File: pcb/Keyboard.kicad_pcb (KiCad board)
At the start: 2 copper layers, 158.5 x 92.5 mm, 63 parts

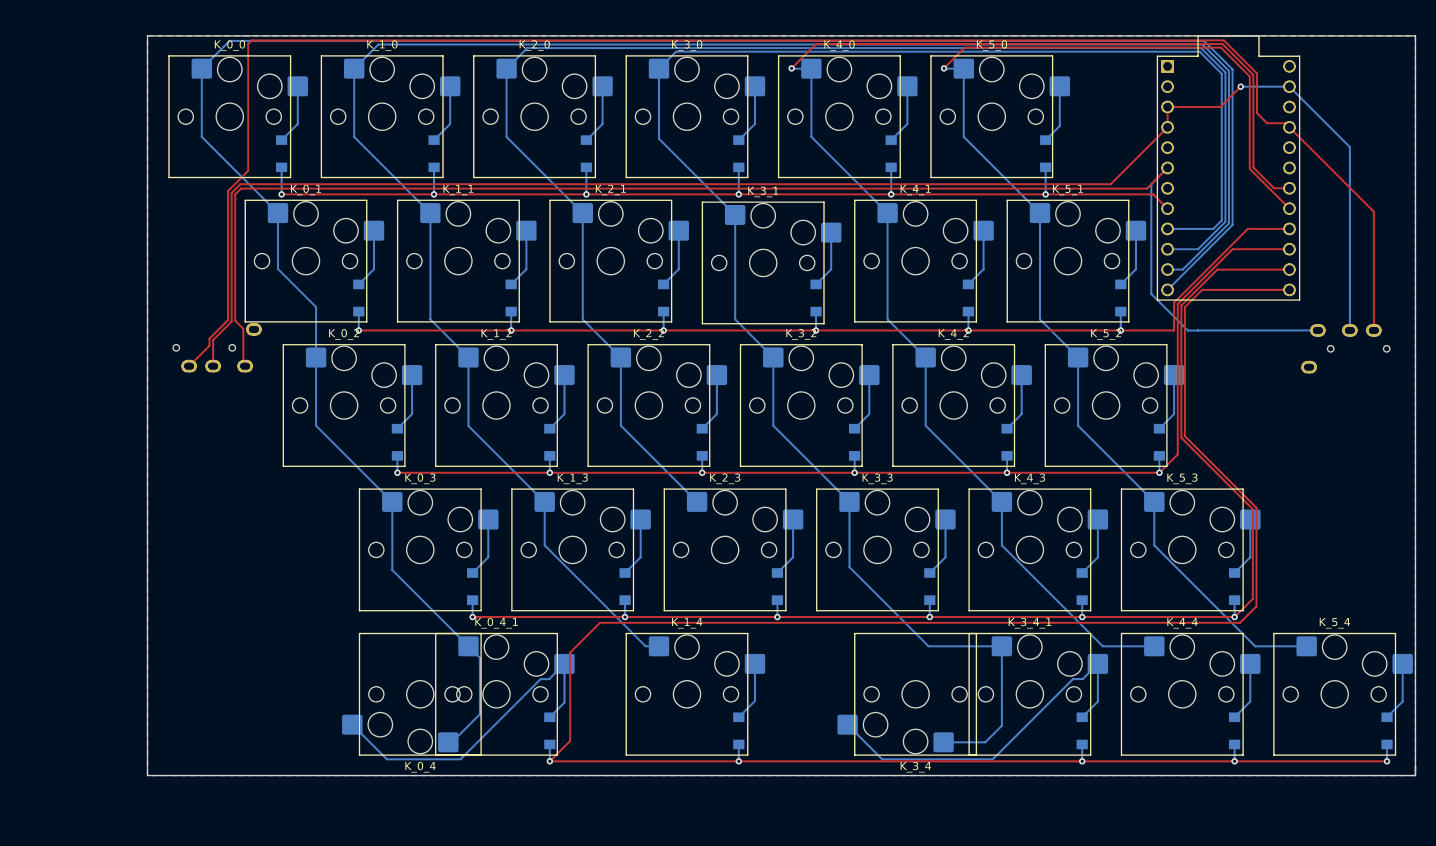
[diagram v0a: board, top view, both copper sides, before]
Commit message: wip
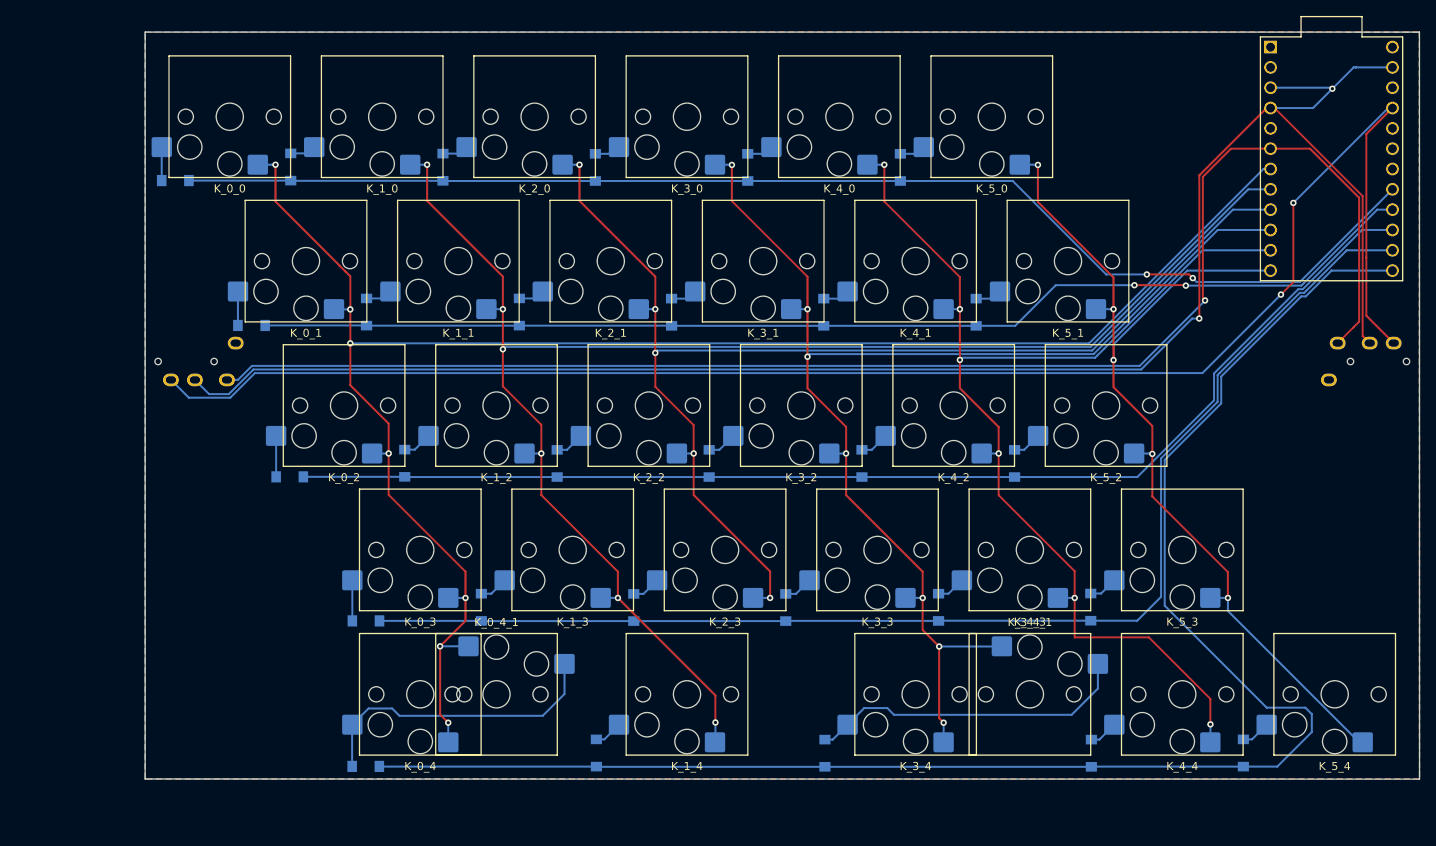
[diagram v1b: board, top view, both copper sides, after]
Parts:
- moved D_3_4 32.3 mm to (141.1, 122.4)
- moved D_0_4 23.4 mm to (83.7, 124.1), turned to 180 degrees
- moved D_3_2 18.4 mm to (126.6, 86.2)
- moved D_2_2 18.3 mm to (107.6, 86.2)
- moved D_4_2 18.3 mm to (145.7, 86.2)
- moved D_1_2 18.3 mm to (88.5, 86.2)
- moved D_5_2 18.3 mm to (164.8, 86.2)
- moved D_5_0 18.2 mm to (150.5, 49.2)
- moved D_3_3 18.2 mm to (136.2, 104.2)
- moved D_4_1 18.2 mm to (140.9, 67.3)
- moved D_5_1 18.2 mm to (160.0, 67.3)
- moved D_5_4 18.2 mm to (193.4, 122.4)
- moved D_1_1 18.2 mm to (83.8, 67.3)
- moved D_5_3 18.2 mm to (174.3, 104.2)
- moved D_2_3 18.1 mm to (117.2, 104.2)
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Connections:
- U_PROMICRO1 pad 10: col2 -> col3
- U_PROMICRO1 pad 11: col1 -> col4
- U_PROMICRO1 pad 12: col0 -> col5
- U_PROMICRO1 pad 17: col5 -> row0
- U_PROMICRO1 pad 18: col4 -> unconnected-(U_PROMICRO1-Pad18)
- U_PROMICRO1 pad 7: unconnected-(U_PROMICRO1-Pad7) -> col0
- U_PROMICRO1 pad 8: row0 -> col1
- U_PROMICRO1 pad 9: col3 -> col2
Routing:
- net row4: track 273.1 -> 203.1 mm, vias 5 -> 0
- net col3: track 211.3 -> 163.9 mm, vias 0 -> 7
- net col0: track 263.2 -> 219.9 mm, vias 0 -> 7
- net col5: track 155.6 -> 123.6 mm, vias 1 -> 5
- net col1: track 230.1 -> 199.8 mm, vias 0 -> 6
- net row0: track 131.8 -> 160.5 mm, vias 6 -> 2
- net col2: track 183.5 -> 156.8 mm, vias 0 -> 5
- net col4: track 173.9 -> 147.4 mm, vias 1 -> 6
- net GND: track 195.4 -> 221.4 mm, vias 1 -> 2
- net row1: track 137.8 -> 147.0 mm, vias 6 -> 2
- net row3: track 166.9 -> 157.9 mm, vias 6 -> 0
- net trrs: track 179.2 -> 184.8 mm, vias 0 -> 1
- net Net-(D_3_4-Pad2): track 45.5 -> 40.5 mm
- net Net-(D_1_0-Pad2): track 7.57 -> 3.25 mm
- net Net-(D_2_0-Pad2): track 7.57 -> 3.29 mm
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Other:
- board size 158.5 x 92.5 mm -> 159.3 x 93.4 mm

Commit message: wip
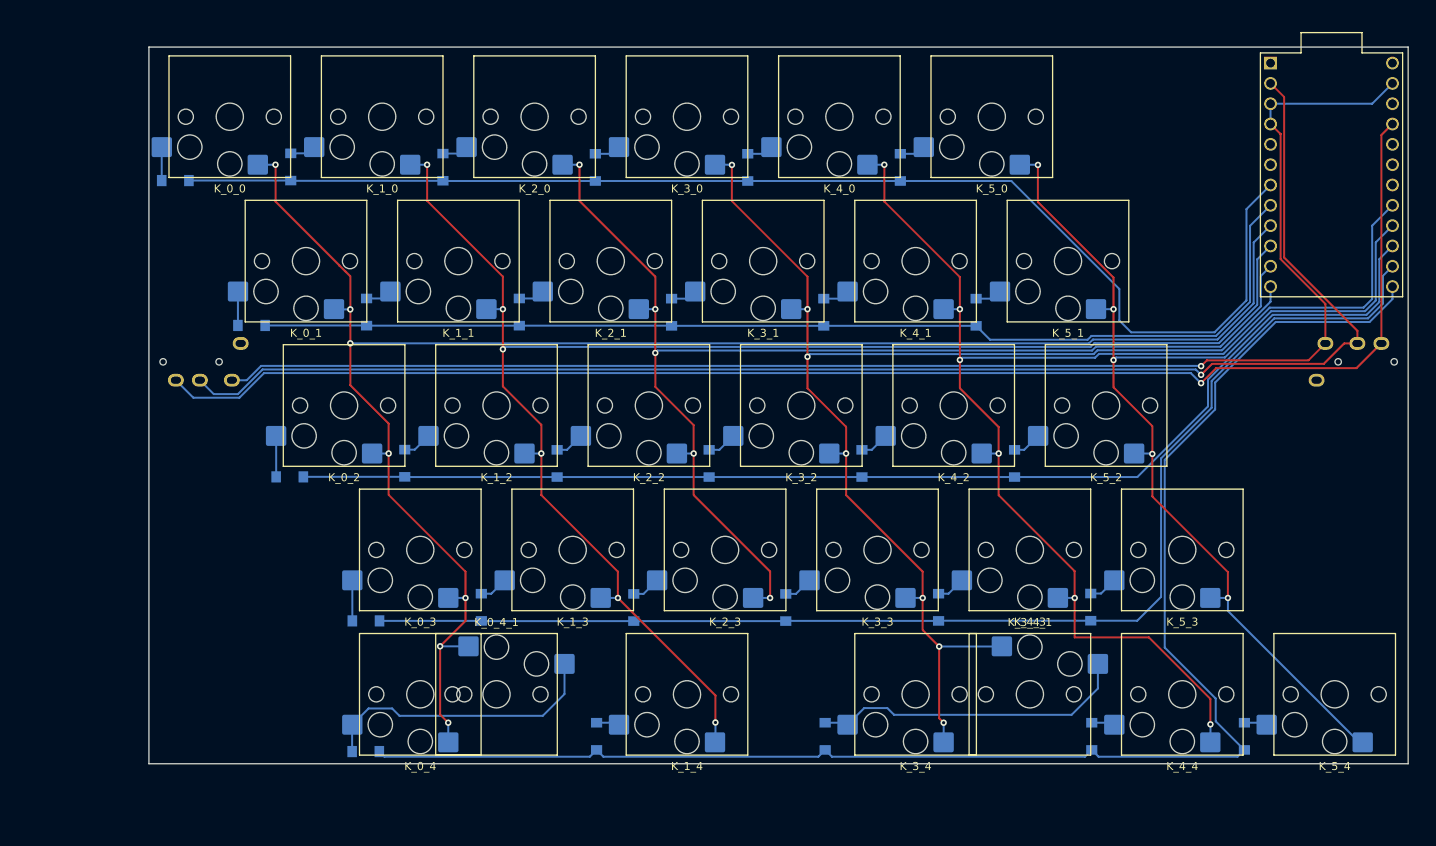
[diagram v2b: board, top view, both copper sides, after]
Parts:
- moved D_4_4 2.11 mm to (174.4, 120.3)
- moved D_3_4 2.11 mm to (141.1, 120.3)
- moved D_5_4 2.09 mm to (193.5, 120.3)
- moved D_1_4 2.08 mm to (112.5, 120.3)
- moved U_PROMICRO1 2.00 mm to (204.4, 50.1)
- moved D_0_4 1.85 mm to (83.7, 122.2)
- moved U_TRRS1 1.54 mm to (213.8, 73.5)
- moved U_TRRS2 0.62 mm to (56.7, 73.5)
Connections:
- U_PROMICRO1 pad 10: col3 -> col1
- U_PROMICRO1 pad 11: col4 -> col2
- U_PROMICRO1 pad 12: col5 -> col3
- U_PROMICRO1 pad 16: row1 -> col5
- U_PROMICRO1 pad 17: row0 -> col4
- U_PROMICRO1 pad 2: unconnected-(U_PROMICRO1-Pad2) -> trrs
- U_PROMICRO1 pad 6: trrs -> unconnected-(U_PROMICRO1-Pad6)
- U_PROMICRO1 pad 7: col0 -> row0
- U_PROMICRO1 pad 8: col1 -> row1
- U_PROMICRO1 pad 9: col2 -> col0
- U_TRRS1 pad 2: trrs -> GND
- U_TRRS1 pad 3: GND -> trrs
- U_TRRS2 pad 2: trrs -> GND
- U_TRRS2 pad 3: GND -> trrs
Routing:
- net GND: track 221.4 -> 187.7 mm, vias 2 -> 1
- net VCC: track 206.6 -> 183.5 mm, vias 2 -> 1
- net col4: track 147.4 -> 170.4 mm
- net col5: track 123.6 -> 144.3 mm
- net row4: track 203.1 -> 191.6 mm
- net row1: track 147.0 -> 138.9 mm, vias 2 -> 0
- net row2: track 150.9 -> 153.2 mm
- net Net-(D_0_4-Pad2): track 37.9 -> 36.0 mm
- net col3: track 163.9 -> 162.0 mm
- net col0: track 219.9 -> 221.4 mm
- net row3: track 157.9 -> 159.1 mm
- net trrs: track 184.8 -> 185.6 mm
- net row0: track 160.5 -> 159.7 mm, vias 2 -> 0
- net Net-(D_5_4-Pad2): track 3.68 -> 2.89 mm
- net Net-(D_4_4-Pad2): track 3.64 -> 2.92 mm
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- removed copper zone on B.Cu, net GND
- removed copper zone on F.Cu, net GND
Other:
- board size 159.3 x 93.4 mm -> 157.4 x 89.6 mm

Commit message: wip
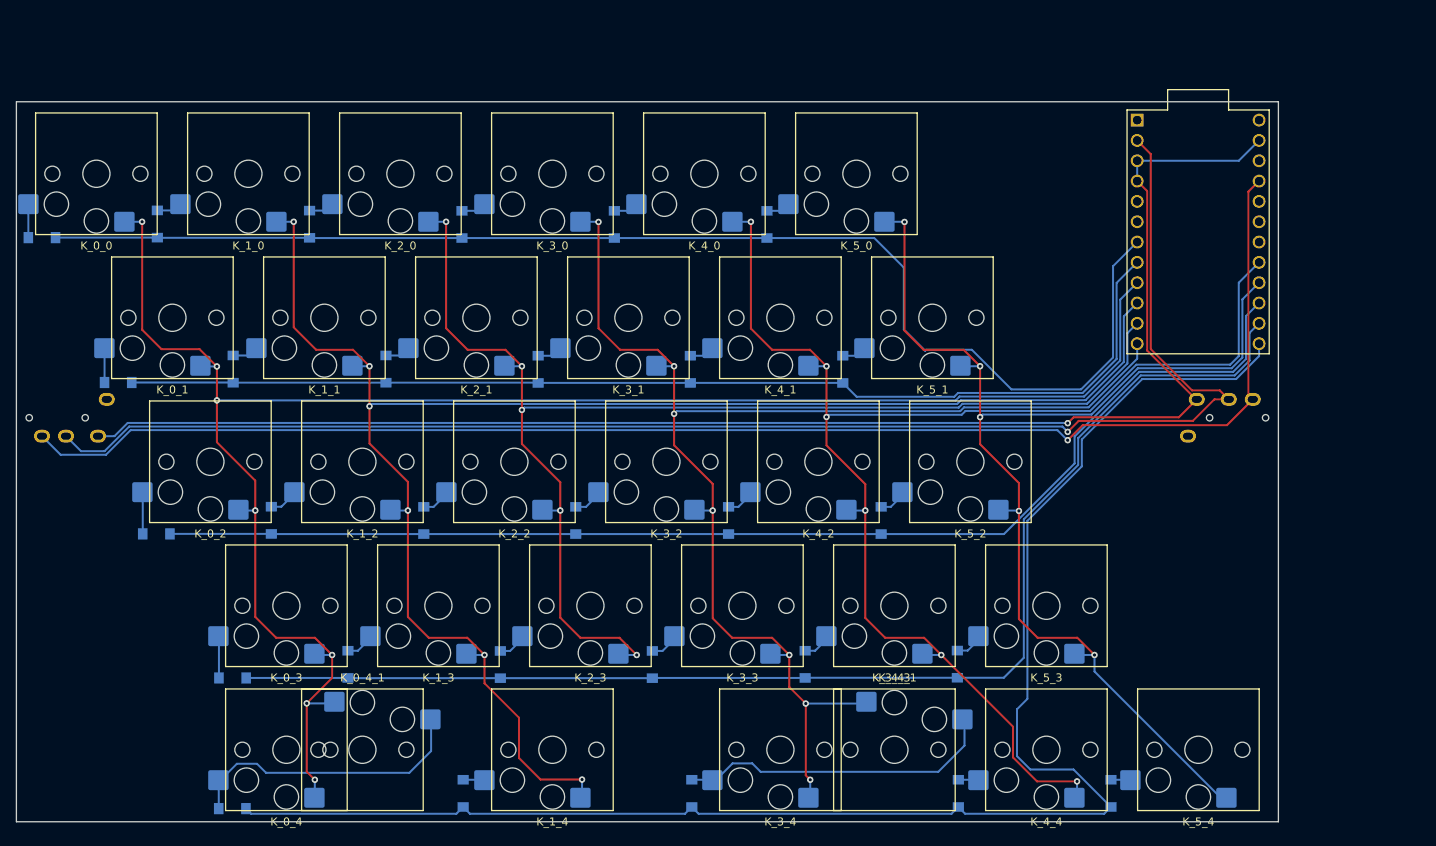
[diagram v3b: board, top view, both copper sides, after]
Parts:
- moved K_5_4 18.4 mm to (187.8, 122.0)
- moved K_5_1 18.4 mm to (154.5, 68.0)
- moved K_5_3 18.4 mm to (168.8, 104.0)
- moved K_5_0 18.4 mm to (145.0, 50.0)
- moved K_5_2 18.4 mm to (159.2, 86.0)
- moved K_4_4 18.3 mm to (168.8, 122.0)
- moved K_4_1 18.3 mm to (135.5, 68.0)
- moved K_4_0 18.3 mm to (126.0, 50.0)
- moved K_4_3 18.3 mm to (149.8, 104.0)
- moved K_4_2 18.3 mm to (140.2, 86.0)
- moved K_3_4_1 18.3 mm to (149.8, 122.0)
- moved K_3_1 18.3 mm to (116.5, 68.0)
- moved K_3_0 18.3 mm to (107.0, 50.0)
- moved K_3_3 18.3 mm to (130.8, 104.0)
- moved K_3_2 18.3 mm to (121.2, 86.0)
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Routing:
- net col1: track 200.2 -> 208.8 mm
- net col5: track 144.3 -> 150.0 mm
- net col2: track 156.0 -> 161.7 mm
- net col3: track 162.0 -> 167.5 mm
- net col0: track 221.4 -> 226.8 mm
- net row4: track 191.6 -> 196.2 mm
- net col4: track 170.4 -> 173.5 mm
- net trrs: track 185.6 -> 188.5 mm
- net row0: track 159.7 -> 162.0 mm
- net VCC: track 183.5 -> 184.3 mm
- net GND: track 187.7 -> 188.5 mm
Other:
- board size 157.4 x 89.6 mm -> 157.8 x 90 mm
